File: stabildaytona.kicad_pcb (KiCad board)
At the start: 4 copper layers, 95 x 79 mm, 95 parts, among them M1 Module-power_12and5V-0.2, M2 Module-knock-0.2, M4 Module-vr-max9924-0.1, U1 TLE9201SG, U10 VNLD5160TR-E, U11 VNLD5160TR-E, U2 TLE9201SG, U4 MAX31855KASA, U6 VNLD5160TR-E, U7 VNLD5160TR-E, U8 VNLD5160TR-E, U9 VNLD5160TR-E

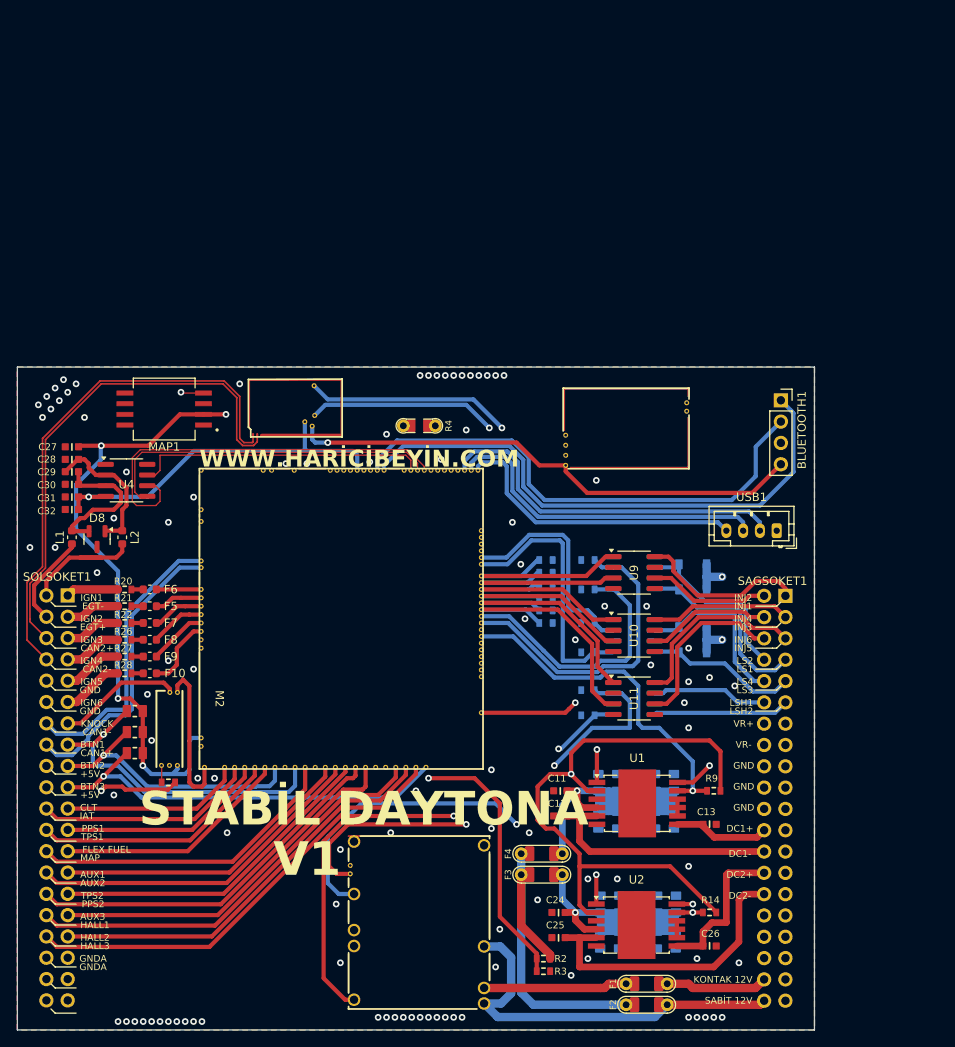
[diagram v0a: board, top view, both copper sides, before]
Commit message: stabil jr.
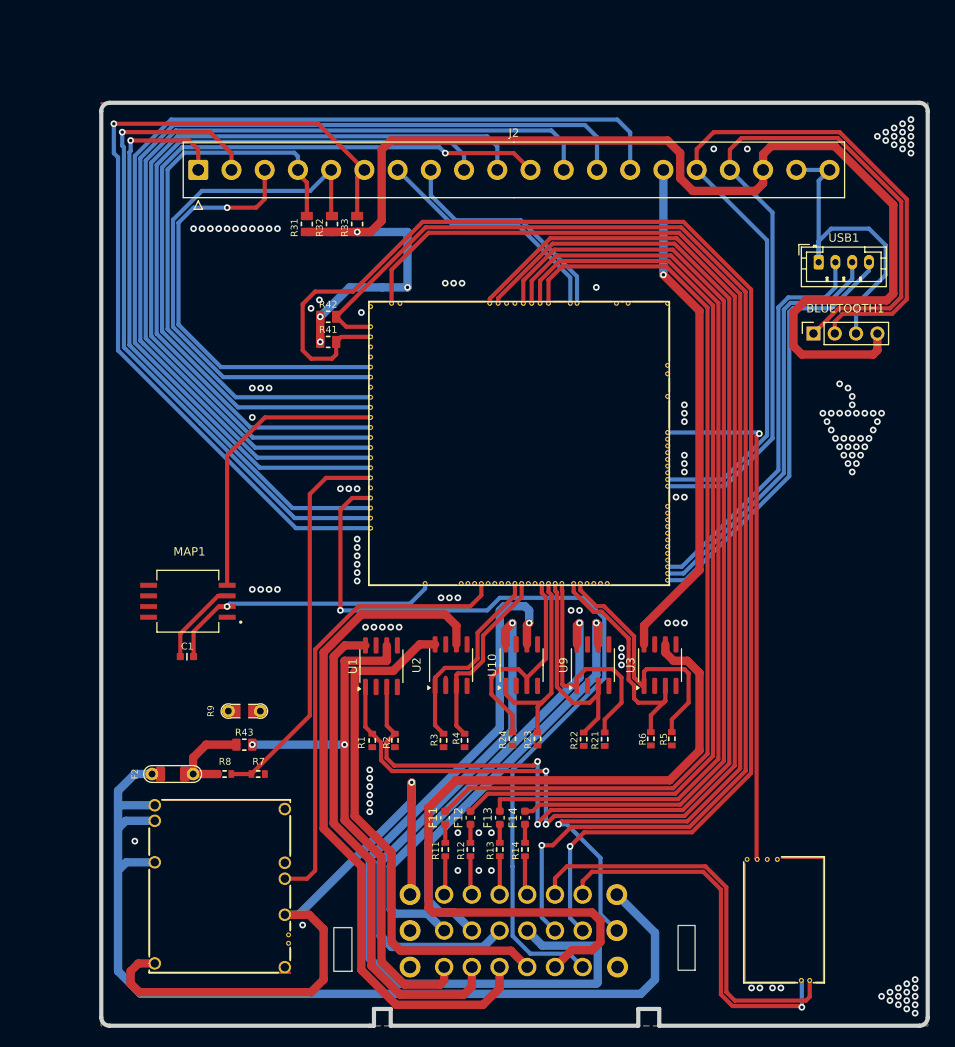
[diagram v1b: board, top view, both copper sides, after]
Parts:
- removed C10, C14, C15, C16, C17, C18, C19, C2, C20, C21, C22, C23, C3, C4, C5, C6, C7, C8, C9: 10u, hellen-one-common:C0805
- removed C11, C24, C27, C29, C31: 100n, hellen-one-common:C0603
- removed C12, C13, C25, C26, C28, C30: 10n, hellen-one-common:C0603
- removed C32: 1u, hellen-one-common:C0603
- removed CAN1: Module-can-0.1, hellen-one-can-0.1:can
- removed D2, D3, D4, D5: B5819W, hellen-one-common:SOD-123
- removed D8: NUP2105L, Package_TO_SOT_SMD:SOT-23
- removed F1, F3, F4: 12H1500D, hellen-one-common:PAD-1206-PAD
- removed F10, F5, F6, F7, F8, F9: 50mA, Fuse:Fuse_0603_1608Metric
- removed L1, L2: 470R@100MHz, Inductor_SMD:L_0603_1608Metric
- removed M2: Module-knock-0.2, hellen-one-knock-0.2:knock
- removed MCU1: Module:mega-mcu100/0.3, hellen-one-mega-mcu100-0.3:mega-mcu100
- removed R10, R15, R16, R29, R30, R34: 4.7k, hellen-one-common:R0603
- removed R20, R26, R27, R28: 0, hellen-one-common:R0603
- removed SAGSOKET1, SOLSOKET1: Conn_02x20_Counter_Clockwise, Connector_PinHeader_2.54mm:PinHeader_2x20_P2.54mm_Vertical
- removed U11, U6, U7, U8: VNLD5160TR-E, Package_SO:SOIC-8_3.9x4.9mm_P1.27mm
- removed U4: MAX31855KASA, Package_SO:SOIC-8_3.9x4.9mm_P1.27mm
- added F11: 50mA, Fuse:Fuse_0603_1608Metric, F.Cu at (101.0, 134.7)
- added F12: 50mA, Fuse:Fuse_0603_1608Metric, F.Cu at (104.0, 134.7)
- added F13: 50mA, Fuse:Fuse_0603_1608Metric, F.Cu at (107.5, 134.7)
- added F14: 50mA, Fuse:Fuse_0603_1608Metric, F.Cu at (110.5, 134.7)
- added J1: Conn_01x24, Connector:24pin, F.Cu at (142.2, 163.3)
- added J2: Conn_01x20, Connector_TE-Connectivity:TE_2-826576-0_1x20_P3.96mm_Vertical, F.Cu at (71.6, 57.5)
- added R1: 4.7k, hellen-one-common:R0603, F.Cu at (92.3, 125.5)
- added R23: 4.7k, hellen-one-common:R0603, F.Cu at (112.0, 125.3)
- added R24: 4.7k, hellen-one-common:R0603, F.Cu at (109.0, 125.3)
- added R41: 2.7K, hellen-one-common:R0805, F.Cu at (87.0, 78.0)
- added R42: 2.7K, hellen-one-common:R0805, F.Cu at (87.0, 75.0)
- added R43: 10K, hellen-one-common:R0805, F.Cu at (77.0, 126.0)
- added U3: VNLD5160TR-E, Package_SO:SOIC-8_3.9x4.9mm_P1.27mm, F.Cu at (126.6, 116.5)
- added İŞLEMC1: Module:mega-mcu100/0.3, hellen-one-mega-mcu100-0.3:mega-mcu100, F.Cu at (91.8, 73.1)
- C1: value 10u -> 100n; footprint hellen-one-common:C0805 -> hellen-one-common:C0603; moved to F.Cu
- MAP1: value MPXH6400A -> GZP6869D200KPP
- R11, R12, R13: value 4.7k -> 0; moved to F.Cu
- R14: value 4.7k -> 0
- R2: value 33k -> 4.7k
- R21, R22, R6: value 0 -> 4.7k
- R3: value 6.8k -> 4.7k
- R31, R32, R33: value 4.7k -> 10k; footprint hellen-one-common:R0603 -> hellen-one-common:R0805; moved to F.Cu
- R4: value Jumper-Pad-Pad -> 4.7k; footprint hellen-one-common:PAD-0805-PAD -> hellen-one-common:R0603
- R5: value 10k -> 4.7k; footprint hellen-one-common:R0805 -> hellen-one-common:R0603
- R7: value 10k -> 6.8k; footprint hellen-one-common:R0805 -> hellen-one-common:R0603
- R8: value 10k -> 33k; footprint hellen-one-common:R0805 -> hellen-one-common:R0603
- R9: value 4.7k -> Jumper-Pad-Pad; footprint hellen-one-common:R0603 -> hellen-one-common:PAD-0805-PAD
- U1, U2: value TLE9201SG -> VNLD5160TR-E; footprint Package_SO:Infineon_PG-DSO-12-11 -> Package_SO:SOIC-8_3.9x4.9mm_P1.27mm
- moved M4 72.9 mm to (146.3, 154.5), turned to 90 degrees
- moved R5 64.1 mm to (128.0, 125.3), turned to -90 degrees
- moved F2 62.8 mm to (68.5, 129.5), turned to 180 degrees
- moved C1 61.2 mm to (70.2, 115.5), turned to 0 degrees
- moved R21 59.4 mm to (120.0, 125.3), turned to 90 degrees
- moved R6 57.7 mm to (125.5, 125.3), turned to -90 degrees
- moved R9 56.8 mm to (77.0, 122.0)
- moved R22 56.4 mm to (117.5, 125.3), turned to 90 degrees
- moved R31 51.6 mm to (84.5, 64.0), turned to -90 degrees
- moved R32 51.3 mm to (87.5, 64.0), turned to -90 degrees
- moved R33 51.3 mm to (90.5, 64.0), turned to -90 degrees
- moved M1 44.0 mm to (65.6, 153.3), turned to 0 degrees
- moved R11 38.5 mm to (101.0, 138.5), turned to 90 degrees
- moved U2 38.1 mm to (101.7, 116.5), turned to 90 degrees
- moved R4 37.9 mm to (103.3, 125.5), turned to -90 degrees
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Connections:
- C1 pad 2: /DC Driver 1/PWR -> +5VA
- M1 pad V2: /IN_VIGN -> +12V_RAW
- M1 pad V4: +5VP -> +5V
- R11 pad 1: GND -> /BOBİN 1
- R11 pad 2: /LS2 -> Net-(F11-Pad1)
- R12 pad 1: GND -> /BOBİN 2
- R12 pad 2: /LS3 -> Net-(F12-Pad1)
- R13 pad 1: GND -> /BOBİN 3
- R13 pad 2: /LS4 -> Net-(F13-Pad1)
- R14 pad 1: /DC2_DIS -> /BOBİN 4
- R14 pad 2: +3.3V -> Net-(F14-Pad1)
- R2 pad 1: /IN_VMAIN -> /AUX GROUP 1/IN1
- R2 pad 2: +12V -> GND
- R21 pad 1: /OUT_IGN2 -> GND
- R21 pad 2: Net-(F5-Pad1) -> /ENJEKTOR/IN1
- R22 pad 1: /OUT_IGN3 -> GND
- R22 pad 2: Net-(F7-Pad1) -> /ENJEKTOR/IN2
- R3 pad 1: GND -> /AUX GROUP 2/IN2
- R3 pad 2: /IN_VMAIN -> GND
- R31 pad 1: GND -> /IN_BUTTON1
- R31 pad 2: /INJ3 -> +5VA
- R32 pad 1: GND -> /IN_BUTTON2
- R32 pad 2: /INJ4 -> +5VA
- R33 pad 1: GND -> /IN_BUTTON3
- R33 pad 2: /INJ5 -> +5VA
- R4 pad 1: Net-(M1-PG_5VP) -> /AUX GROUP 2/IN1
- R4 pad 2: /PG_5VP -> GND
- R5 pad 1: /IN_BUTTON1 -> /AUX GROUP 3/IN2
- R5 pad 2: +5VA -> GND
- R6 pad 1: /IN_KNOCK -> /AUX GROUP 3/IN1
- R6 pad 2: /ADC3 -> GND
- R7 pad 1: /IN_BUTTON2 -> GND
- R7 pad 2: +5VA -> /IN_VMAIN
- R8 pad 1: /IN_BUTTON3 -> /IN_VMAIN
- R8 pad 2: +5VA -> +12V
- R9 pad 1: /DC1_DIS -> Net-(M1-PG_5VP)
- R9 pad 2: +3.3V -> /PG_5VP
- U1 pad 1: /DC1_DIR -> /AUX GROUP 1/IN2
- U1 pad 2: +3.3V -> unconnected-(U1-STATUS1-Pad2)
- U1 pad 3: unconnected-(U1-SO-Pad3) -> /AUX GROUP 1/IN1
- U1 pad 4: /DC Driver 1/PWR -> unconnected-(U1-STATUS2-Pad4)
- U1 pad 5: /OUT_DC1- -> GND
- U1 pad 6: GND -> /ÇIKIŞ 1
- U1 pad 7: /OUT_DC1+ -> GND
- U1 pad 8: GND -> /ÇIKIŞ 2
- U10 pad 1: /INJ3 -> /ENJEKTOR/IN3
- U10 pad 3: /INJ4 -> /ENJEKTOR/IN4
- U10 pad 6: /OUT_INJ4 -> /ENJEKTÖR 4
- U10 pad 8: /OUT_INJ3 -> /ENJEKTÖR 3
- U2 pad 1: /DC2_DIR -> /AUX GROUP 2/IN2
- U2 pad 2: +3.3V -> unconnected-(U2-STATUS1-Pad2)
- U2 pad 3: unconnected-(U2-SO-Pad3) -> /AUX GROUP 2/IN1
- U2 pad 4: /DC Driver 2/PWR -> unconnected-(U2-STATUS2-Pad4)
- U2 pad 5: /OUT_DC2- -> GND
- U2 pad 6: GND -> /ÇIKIŞ 3
- U2 pad 7: /OUT_DC2+ -> GND
- U2 pad 8: GND -> /ÇIKIŞ 4
- U9 pad 1: /INJ1 -> /ENJEKTOR/IN1
- U9 pad 3: /INJ2 -> /ENJEKTOR/IN2
- U9 pad 6: /OUT_INJ2 -> /ENJEKTÖR 2
- U9 pad 8: /OUT_INJ1 -> /ENJEKTÖR 1
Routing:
- net +3.3V: track 155.6 -> 0.00 mm, vias 1 -> 0
- net /AUX GROUP 1/IN2: track 0.00 -> 153.0 mm, vias 0 -> 2
- net /AUX GROUP 1/IN1: track 0.00 -> 150.3 mm, vias 0 -> 2
- net /IN_IAT: track 26.3 -> 170.3 mm, vias 0 -> 1
- net /PG_5VP: track 5.38 -> 142.3 mm
- net /IN_CLT: track 21.7 -> 156.9 mm, vias 0 -> 1
- net /ANALOG 8: track 0.00 -> 122.5 mm
- net +5VA: track 192.4 -> 308.5 mm, vias 6 -> 5
- net /ANALOG 7: track 0.00 -> 115.6 mm
- net /BOBIN/IN3: track 0.00 -> 112.3 mm
- net /BOBIN/IN2: track 0.00 -> 111.8 mm
- net /BOBIN/IN1: track 0.00 -> 111.7 mm
- net /BOBIN/IN4: track 0.00 -> 111.7 mm
- net /DC Driver 1/PWR: track 110.2 -> 0.00 mm, vias 1 -> 0
- net /ANALOG 6: track 0.00 -> 108.5 mm
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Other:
- board size 95 x 79 mm -> 98.5 x 110 mm
- board text added: "STABİL JR."
- board text added: "ÖZER"
- board text removed: "+5V"
- board text removed: "AUX1"
- board text removed: "AUX2"
- board text removed: "AUX3"
- board text removed: "BTN1"
- board text removed: "BTN2"
- board text removed: "BTN3"
- board text removed: "CAN1+"
- board text removed: "CAN1-"
- board text removed: "CAN2+"
- board text removed: "CAN2-"
- board text removed: "CLT"
- board text removed: "DC1+"
- board text removed: "DC1-"
- board text removed: "DC2+"
- board text removed: "DC2-"
- board text removed: "EGT+"
- board text removed: "EGT-"
- board text removed: "FLEX FUEL"
- board text removed: "GND"
- board text removed: "GNDA"
- board text removed: "HALL1"
- board text removed: "HALL2"
- board text removed: "HALL3"
- board text removed: "IAT"
- board text removed: "IGN1"
- board text removed: "IGN2"
- board text removed: "IGN3"
- board text removed: "IGN4"
- board text removed: "IGN5"
- board text removed: "IGN6"
- board text removed: "INJ1"
- board text removed: "INJ2"
- board text removed: "INJ3"
- board text removed: "INJ4"
- board text removed: "INJ5"
- board text removed: "INJ6"
- board text removed: "KNOCK"
- board text removed: "KONTAK 12V"
- board text removed: "LS1"
- board text removed: "LS2"
- board text removed: "LS3"
- board text removed: "LS4"
- board text removed: "LSH1"
- board text removed: "LSH2"
- board text removed: "MAP"
- board text removed: "PPS1"
- board text removed: "PPS2"
- board text removed: "SABİT 12V"
- board text removed: "STABİL DAYTONA"
- board text removed: "TPS1"
- board text removed: "TPS2"
- board text removed: "V1"
- board text removed: "VR+"
- board text removed: "VR-"
- board text removed: "WWW.HARİCİBEYİN.COM"

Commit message: v2
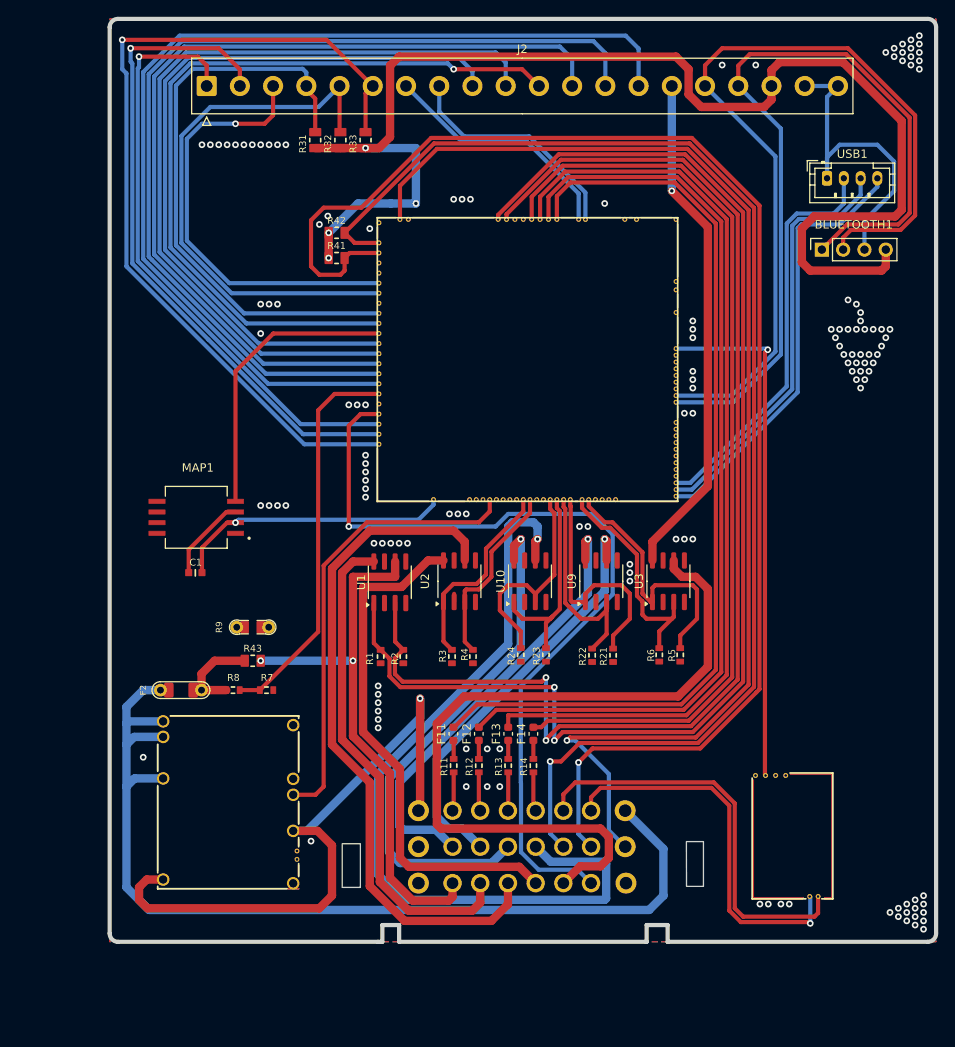
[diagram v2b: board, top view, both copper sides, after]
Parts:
- moved BLUETOOTH1 10.0 mm to (145.9, 67.0)
- moved C1 10.0 mm to (71.2, 105.5)
- moved F11 10.0 mm to (102.0, 124.7)
- moved F12 10.0 mm to (105.0, 124.7)
- moved F13 10.0 mm to (108.5, 124.7)
- moved F14 10.0 mm to (111.5, 124.7)
- moved F2 10.0 mm to (69.5, 119.5)
- moved J1 10.0 mm to (143.2, 153.3)
- moved J2 10.0 mm to (72.6, 47.5)
- moved M1 10.0 mm to (66.6, 143.3)
- moved M4 10.0 mm to (147.3, 144.5)
- moved MAP1 10.0 mm to (71.3, 98.9)
- moved R1 10.0 mm to (93.3, 115.5)
- moved R11 10.0 mm to (102.0, 128.5)
- moved R12 10.0 mm to (105.0, 128.5)
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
